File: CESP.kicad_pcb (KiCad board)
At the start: 2 copper layers, 55.9 x 44.7 mm, 9 parts

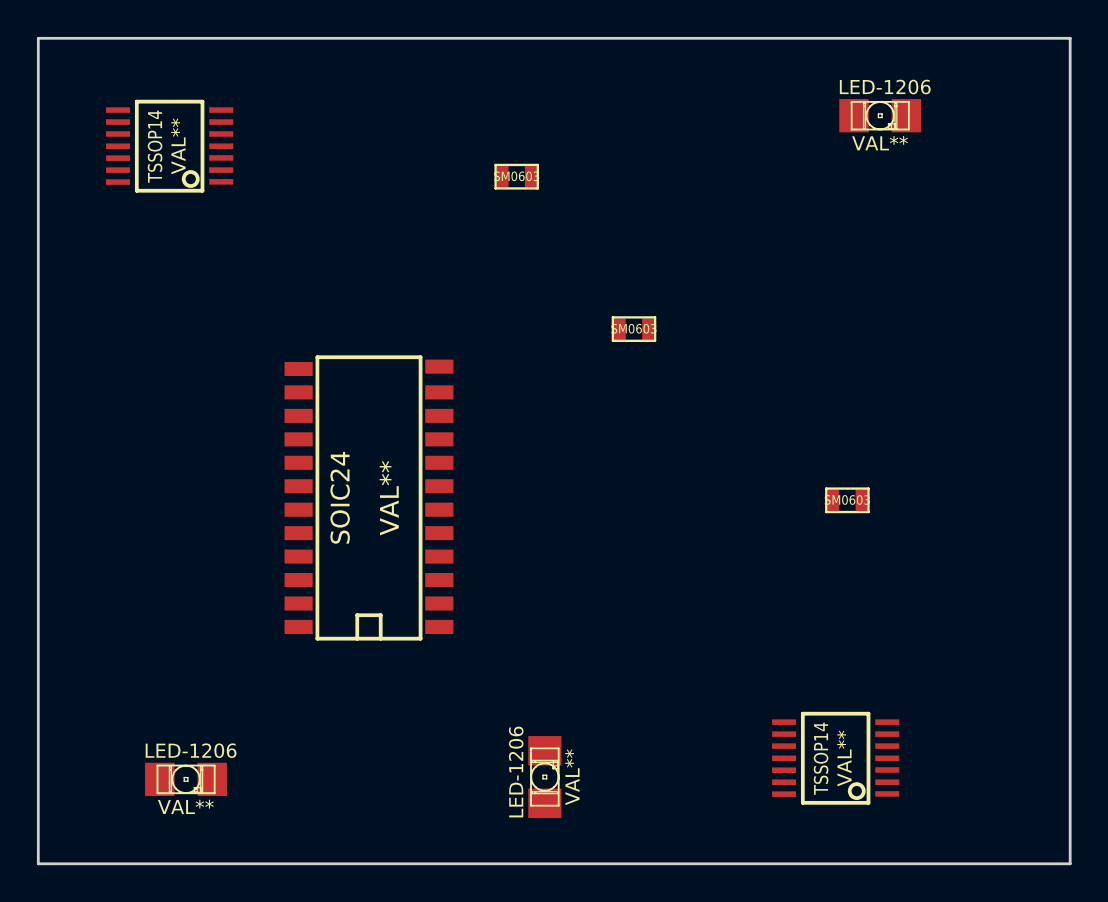
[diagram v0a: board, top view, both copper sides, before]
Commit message: modified:   CESP-cache.lib new file:   CESP.cmp modified:   CESP.kicad_pcb modified:   CESP.kicad_pcb-bak new file:   CESP.net modified:   CESP.pro modified:   CESP.sch new file:   GLSP.lib new file:   GLSP.pretty/DPAK3.kicad_mod new file:   GLSP.pretty/FDMC8360L.kicad_mod new file:   GLSP.pretty/MCP6002.kicad_mod new file:   GLSP.pretty/TB62752AFUG.kicad_mod new file:   GLSP.pretty/ZXBM1021.kicad_mod new file:   Gerber/CESP-B_Cu.gbl new file:   Gerber/CESP-B_SilkS.gbo new file:   Gerber/CESP-F_Cu.gtl new file:   Gerber/CESP-F_SilkS.gto new file:   Gerber/CESP.drl new file:   fp-lib-table new file:   images/snapshot1.png new file:   images/snapshot2.png new file:   images/snapshot3.png
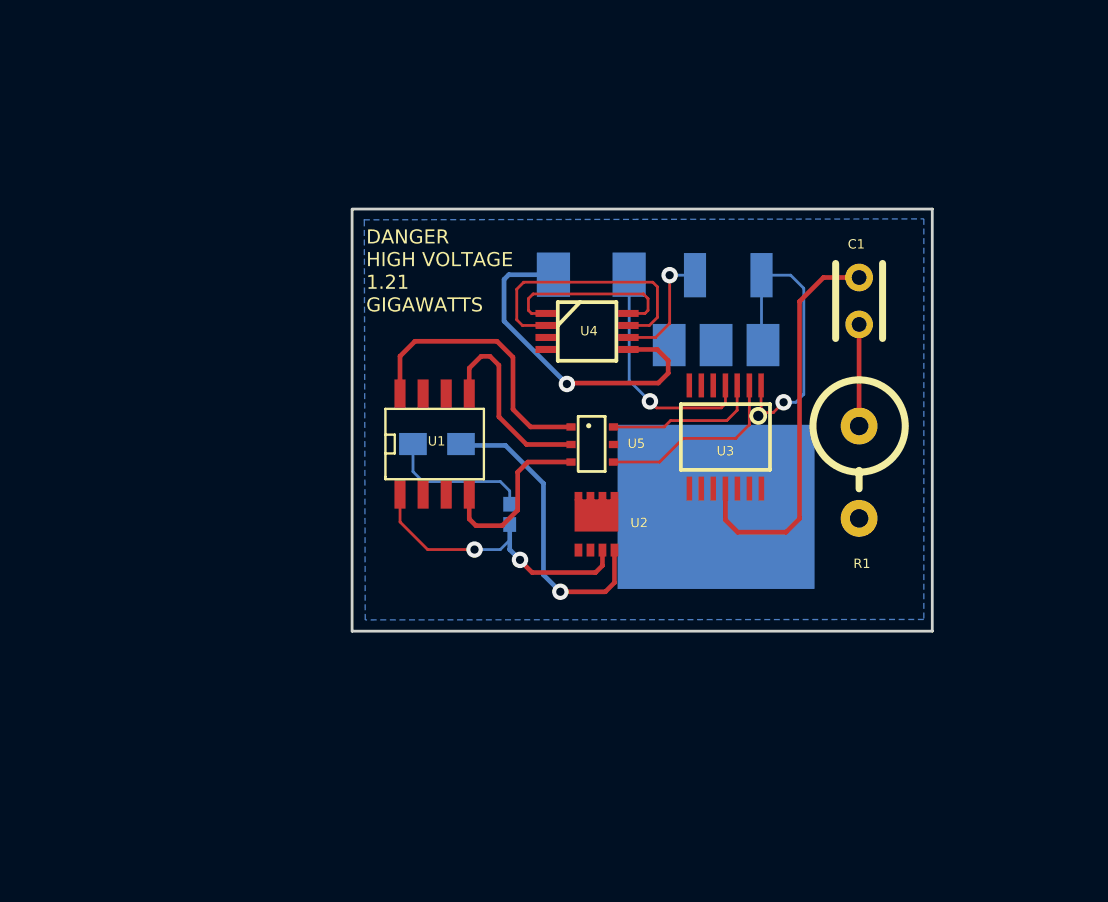
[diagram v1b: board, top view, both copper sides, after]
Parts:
- removed LED-1206 (x3): VAL**, LED-1206
- removed SM0603 (x3): Val**, SM0603
- removed SOIC24: VAL**, SOIC24
- removed TSSOP14 (x2): VAL**, TSSOP14
- added C1: C, Capacitors_ThroughHole:Capacitor4x3RM2.5, F.Cu at (200.4, 108.7)
- added C3: C, Capacitors_SMD:c_0402, B.Cu at (181.5, 121.5)
- added C4: C, Capacitors_SMD:c_1808, B.Cu at (185.9, 108.6)
- added R1: R, Resistors_ThroughHole:Resistor_Vertical_RM5mm, F.Cu at (200.4, 119.3)
- added R3: R, Resistors_SMD:Resistor_SMD0805_HandSoldering, B.Cu at (177.5, 117.7)
- added R4: R, Resistors_SMD:Resistor_SMD1210_ReflowWave, B.Cu at (193.3, 108.6)
- added U1: AO4576, SOIC_Packages:SOIC-8_N, F.Cu at (177.4, 117.7)
- added U2: FDMC8360L, GLSP:FDMC8360L, F.Cu at (186.2, 122.1)
- added U3: LM324, SMD_Packages:TSSOP14, F.Cu at (193.2, 117.3)
- added U4: MCP6002, SMD_Packages:MSOP_8, F.Cu at (185.7, 111.6)
- added U5: TB62752AFUG, GLSP:TB62752AFUG, F.Cu at (186.0, 117.8)
- added U6: 7805, GLSP:DPAK3, B.Cu at (192.7, 112.4)
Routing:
- net Net-(C1-Pad1): track 0.00 -> 21.8 mm
- net Net-(C4-Pad1): track 0.00 -> 18.8 mm, vias 0 -> 1
- net Net-(C3-Pad1): track 0.00 -> 17.0 mm, vias 0 -> 2
- net Net-(R3-Pad2): track 0.00 -> 16.5 mm, vias 0 -> 1
- net Net-(R4-Pad2): track 0.00 -> 16.2 mm, vias 0 -> 1
- net Net-(U1-Pad8): track 0.00 -> 15.2 mm
- net Net-(U4-Pad2): track 0.00 -> 14.8 mm
- net Net-(C4-Pad2): track 0.00 -> 12.6 mm, vias 0 -> 1
- net Net-(U1-Pad5): track 0.00 -> 10.8 mm
- net Net-(U3-Pad2): track 0.00 -> 10.3 mm
- net Net-(U4-Pad1): track 0.00 -> 10.3 mm
- net Net-(U1-Pad4): track 0.00 -> 9.65 mm
- net Net-(U3-Pad3): track 0.00 -> 8.42 mm
- net Net-(C3-Pad2): track 0.00 -> 7.89 mm
- net Net-(R4-Pad1): track 0.00 -> 6.62 mm, vias 0 -> 1
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- added copper zone on B.Cu, net GND
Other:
- board size 55.9 x 44.7 mm -> 31.4 x 22.9 mm
- rule trace_min: 0.254 -> 0.1524
- rule via_min_drill: 0.508 -> 0.127
- rule via_min_size: 0.889 -> 0.254
- board text added: "DANGER HIGH VOLTAGE 1.21 GIGAWATTS"
- board text added: "GL"
- board text removed: "NOTE: THIS IS JUST A TEST BOARD REMOVE ALL COMPONENTS AND CREATE YOUR OWN INCLUDE SCHEMATIC HOOKUPS/NETLIST"
